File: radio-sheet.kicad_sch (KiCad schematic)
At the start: 43 parts, among them Q2 AO3401A, Q3 MMBT3904, Q4 AO3401A, U15 74HC04, U5 Si4463, Y4 30M

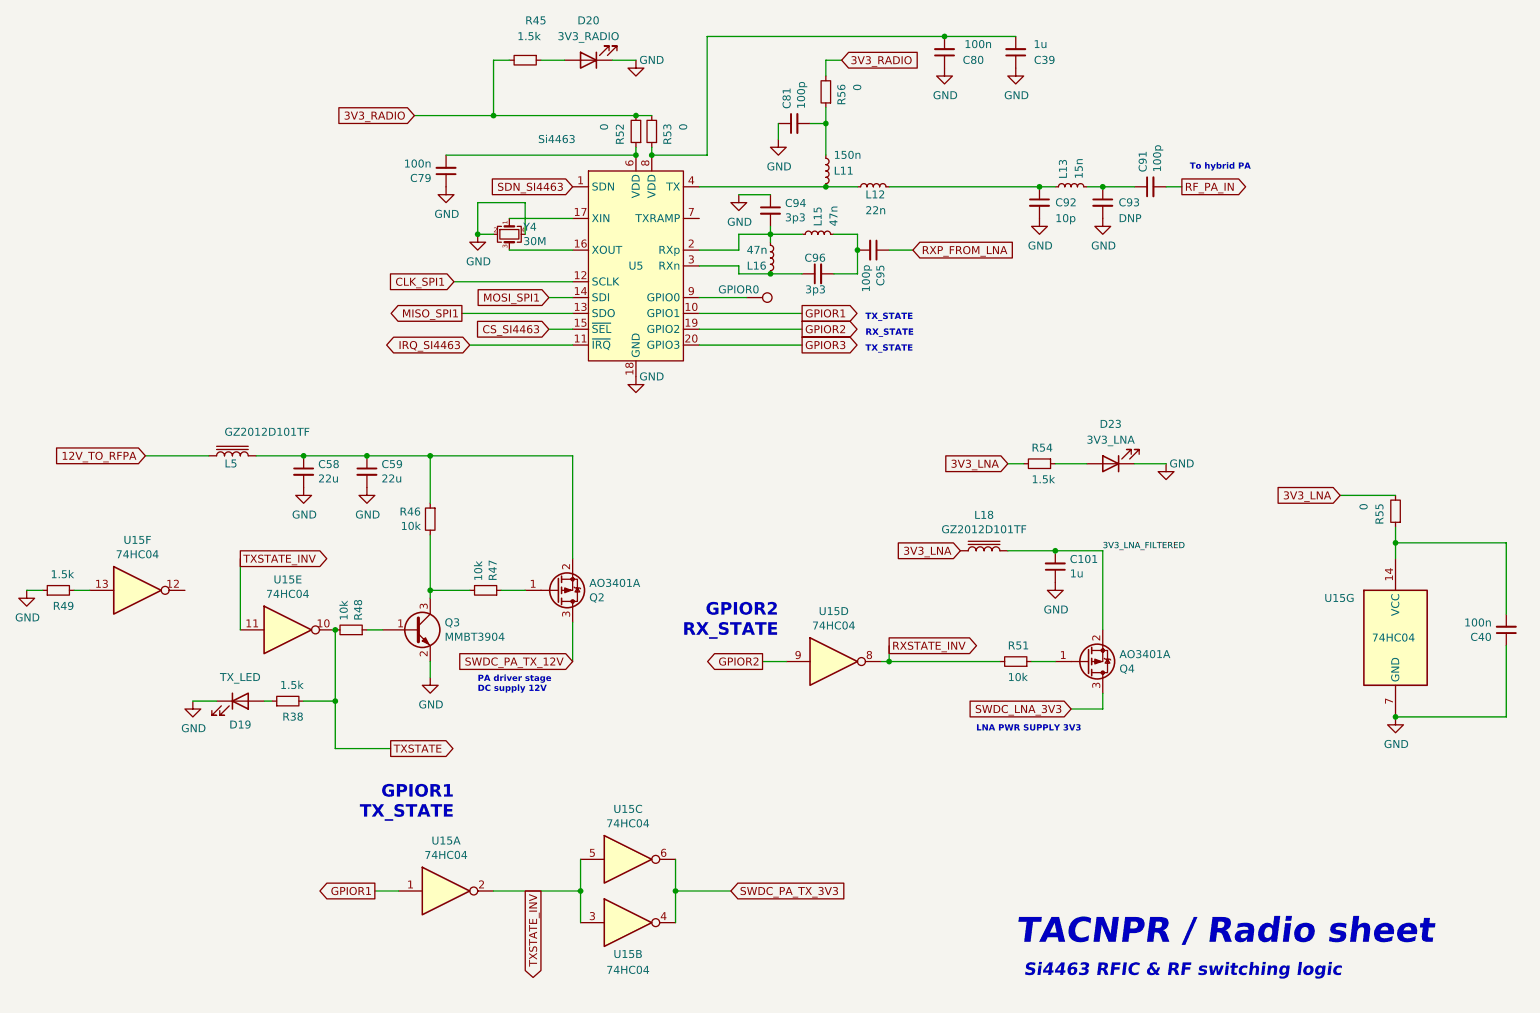
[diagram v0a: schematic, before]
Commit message: misc
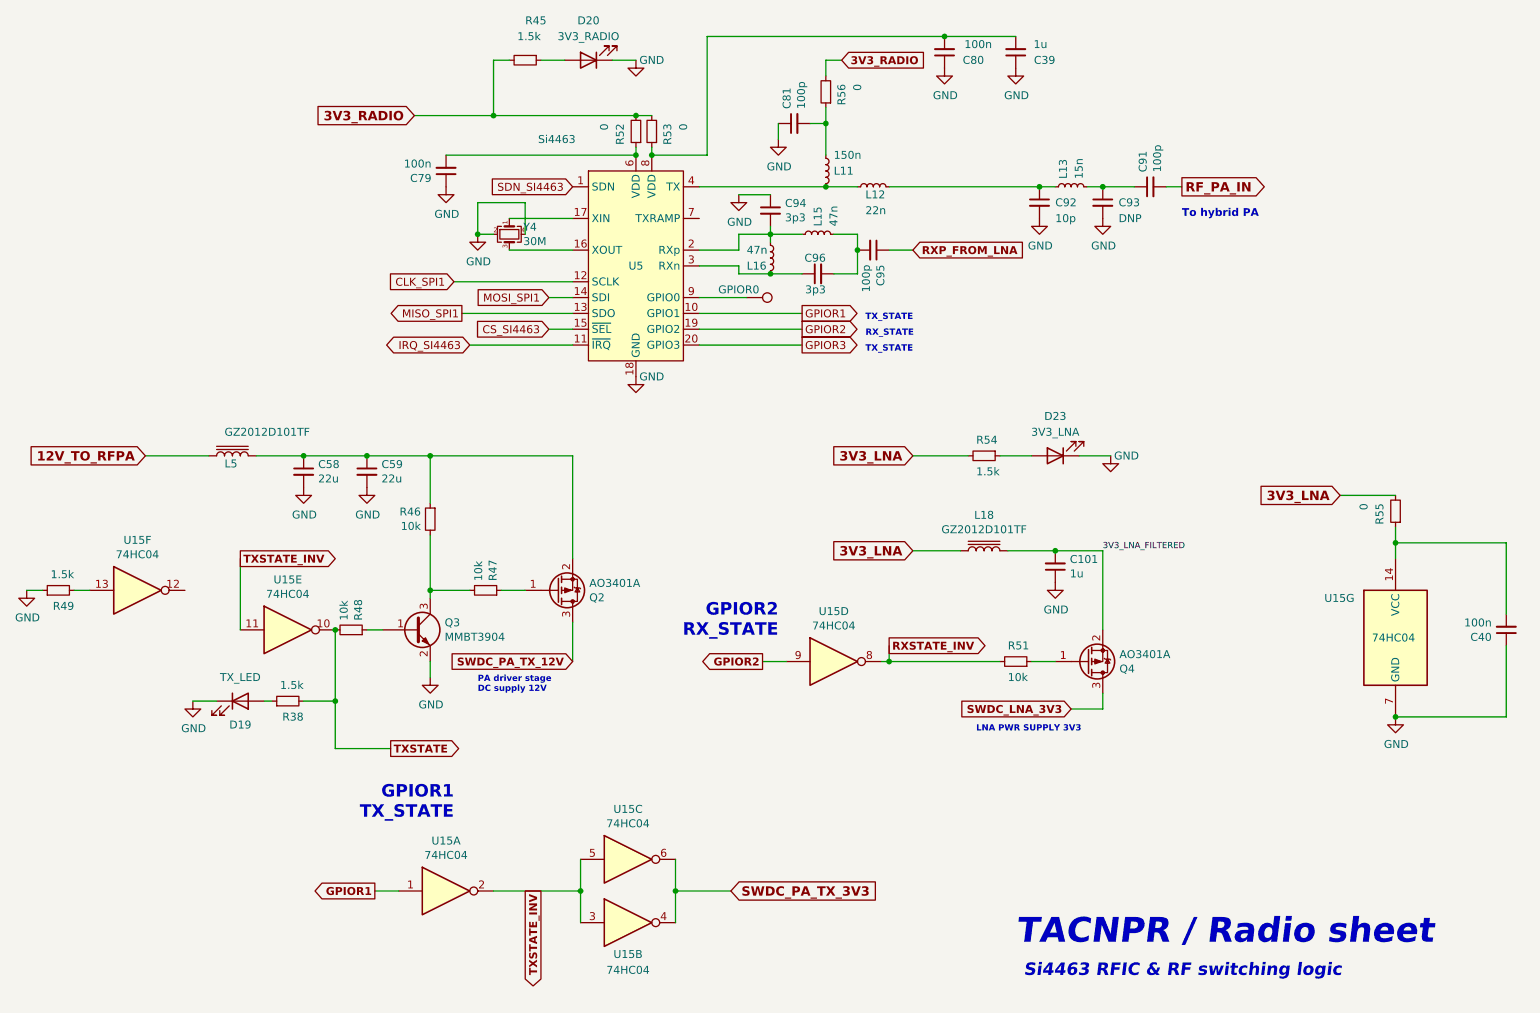
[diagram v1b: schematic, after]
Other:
- moved on the sheet: D23, R54
